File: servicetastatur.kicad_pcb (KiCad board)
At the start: 2 copper layers, 113.9 x 58 mm, 70 parts, among them J1 Conn_01x02, J2 LCD, J3 Automat, J4 Tasten, J5 Conn_01x03_Pin, J6 Conn_01x03_Pin, Q1 2N3904, U1 74HC238, U17 TL7705A, U18 MC34063AP, U2 74HC00, U3 27C128, U4 80C31, U5 74LS573, U6 74HC4094, U7 74HC4094, U8 74HC165, U9 24CS16, Y1 11.059

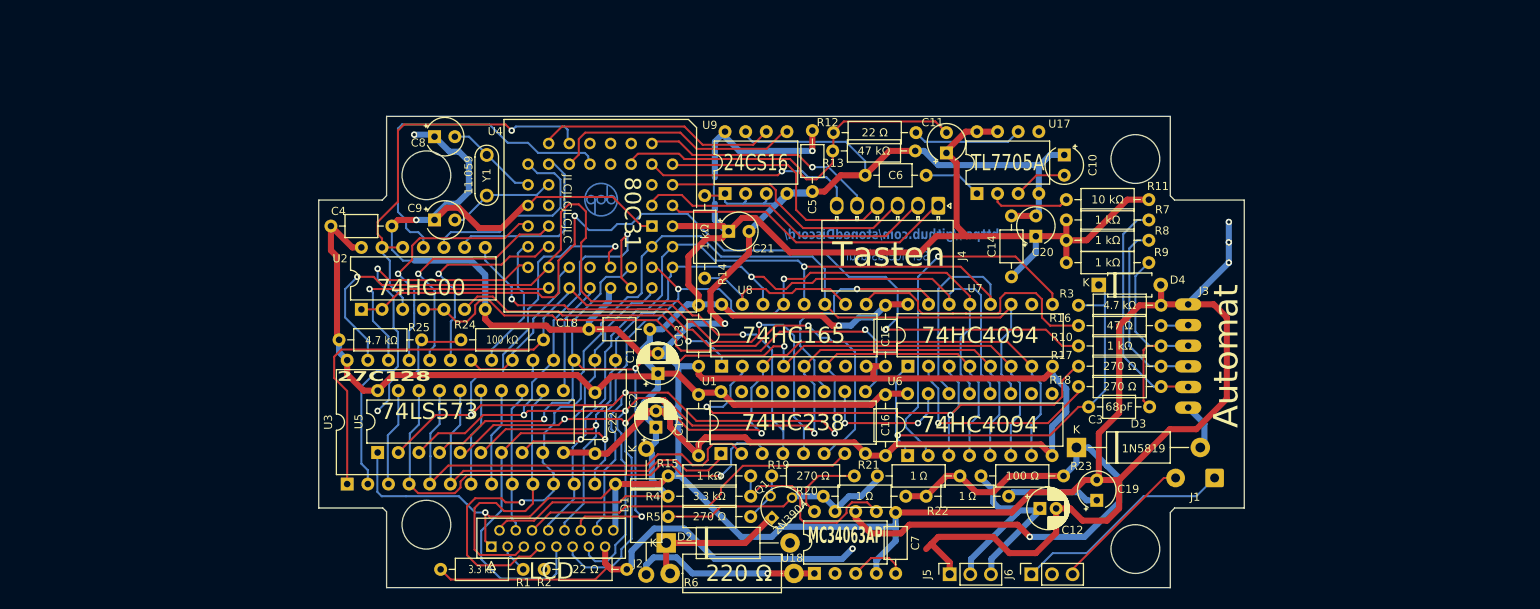
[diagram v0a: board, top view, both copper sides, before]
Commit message: kompakt
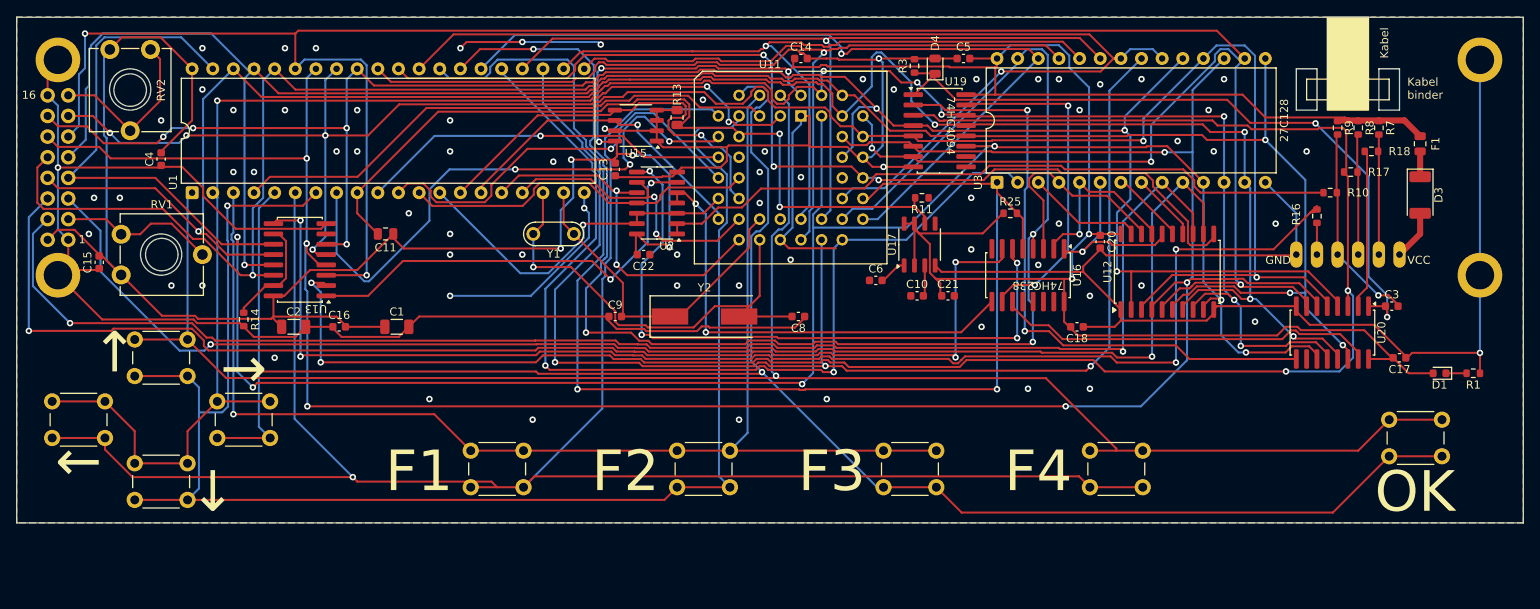
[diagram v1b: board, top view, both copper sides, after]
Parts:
- removed C12: C_Polarized, Capacitor_THT:CP_Radial_D5.0mm_P2.00mm
- removed C19: C, Capacitor_THT:CP_Radial_Tantal_D4.5mm_P2.50mm
- removed C7: C, Capacitor_THT:C_Axial_L3.8mm_D2.6mm_P7.50mm_Horizontal
- removed D2: D, Diode_THT:D_DO-15_P15.24mm_Horizontal
- removed J1: Conn_01x02, Connector_Wire:SolderWire-0.5sqmm_1x02_P4.8mm_D0.9mm_OD2.3mm
- removed J4: Tasten, adp:FFC_1x06_P2.50mm_Horizontal
- removed J5, J6: Conn_01x03_Pin, Connector_PinSocket_2.54mm:PinSocket_1x03_P2.54mm_Vertical
- removed Q1: 2N3904, adp:TO-92
- removed R12, R2: 22 Ω, Resistor_THT:R_Axial_DIN0207_L6.3mm_D2.5mm_P10.16mm_Horizontal
- removed R15: 1 kΩ, Resistor_THT:R_Axial_DIN0207_L6.3mm_D2.5mm_P10.16mm_Horizontal
- removed R19, R5: 270 Ω, Resistor_THT:R_Axial_DIN0207_L6.3mm_D2.5mm_P10.16mm_Horizontal
- removed R20, R21, R22: 1 Ω, Resistor_THT:R_Axial_DIN0207_L6.3mm_D2.5mm_P10.16mm_Horizontal
- removed R23: 100 Ω, Resistor_THT:R_Axial_DIN0207_L6.3mm_D2.5mm_P10.16mm_Horizontal
- removed R24: 100 kΩ, Resistor_THT:R_Axial_DIN0207_L6.3mm_D2.5mm_P10.16mm_Horizontal
- removed R4: 3.3 kΩ, Resistor_THT:R_Axial_DIN0207_L6.3mm_D2.5mm_P10.16mm_Horizontal
- removed R6: 220 Ω, Resistor_THT:R_Axial_DIN0414_L11.9mm_D4.5mm_P15.24mm_Horizontal
- removed U18: MC34063AP, Package_DIP:DIP-8_W7.62mm
- removed U4: 80C31, Package_LCC:PLCC-44_THT-Socket
- removed U5: 74LS573, Package_DIP:DIP-20_W7.62mm
- removed U6, U7: 74HC4094, Package_DIP:DIP-16_W7.62mm
- removed U8: 74HC165, Package_DIP:DIP-16_W7.62mm
- removed U9: 24CS16, Package_DIP:DIP-8_W7.62mm
- added F1: Fuse, Fuse:Fuse_0805_2012Metric, F.Cu at (185.4, 34.6)
- added RV1: Kontrast, Potentiometer_THT:Potentiometer_ACP_CA9-V10_Vertical_Hole, F.Cu at (25.6, 50.8)
- added RV2: Helligkeit, Potentiometer_THT:Potentiometer_ACP_CA9-V10_Vertical_Hole, F.Cu at (24.2, 23.0)
- added SW1: OK, Button_Switch_THT:SW_PUSH_6mm, F.Cu at (181.6, 68.6)
- added SW2: →, Button_Switch_THT:SW_PUSH_6mm, F.Cu at (37.4, 66.3)
- added SW3: F3, Button_Switch_THT:SW_PUSH_6mm, F.Cu at (119.4, 72.4)
- added SW4: F4, Button_Switch_THT:SW_PUSH_6mm, F.Cu at (144.8, 72.4)
- added SW5: ←, Button_Switch_THT:SW_PUSH_6mm, F.Cu at (17.1, 66.3)
- added SW6: F1, Button_Switch_THT:SW_PUSH_6mm, F.Cu at (68.6, 72.4)
- added SW7: ↑, Button_Switch_THT:SW_PUSH_6mm, F.Cu at (27.2, 58.7)
- added SW8: ↓, Button_Switch_THT:SW_PUSH_6mm, F.Cu at (27.2, 74.0)
- added SW9: F2, Button_Switch_THT:SW_PUSH_6mm, F.Cu at (94.0, 72.4)
- added U11: 80C31, Package_LCC:PLCC-44_THT-Socket, F.Cu at (109.2, 31.2)
- added U12: 74LS573, Package_SO:SOIC-20W_7.5x12.8mm_P1.27mm, F.Cu at (154.3, 50.4)
- added U13: 74HC165, Package_SO:SOIC-16W_5.3x10.2mm_P1.27mm, F.Cu at (47.5, 48.9)
- added U15: 24CS16, Package_SO:SO-8_3.9x4.9mm_P1.27mm, F.Cu at (88.9, 32.4)
- added U16: 74HC238, Package_SO:SOIC-16W_5.3x10.2mm_P1.27mm, F.Cu at (137.2, 50.8)
- added U19: 74HC4094, Package_SO:SOIC-16W_5.3x10.2mm_P1.27mm, F.Cu at (126.3, 33.0)
- added U20: 74HC4094, Package_SO:SOIC-16W_5.3x10.2mm_P1.27mm, F.Cu at (174.6, 57.9)
- added Y2: 11.059, Crystal:Crystal_SMD_HC49-SD, F.Cu at (97.3, 55.9)
- C1: value C_Polarized -> 1uF; footprint Capacitor_THT:CP_Radial_D5.0mm_P2.50mm -> Capacitor_SMD:C_1206_3216Metric
- C10: value C -> 0,1uF; footprint Capacitor_THT:CP_Radial_Tantal_D4.5mm_P2.50mm -> Capacitor_SMD:C_0603_1608Metric
- C11: footprint Capacitor_THT:CP_Radial_Tantal_D4.5mm_P2.50mm -> Capacitor_SMD:C_0805_2012Metric
- C13, C14, C15, C16, C17, C18, C22, C5: value C -> 100nF; footprint Capacitor_THT:C_Axial_L3.8mm_D2.6mm_P7.50mm_Horizontal -> Capacitor_SMD:C_0603_1608Metric
- C2: value C_Polarized -> 1uF; footprint Capacitor_THT:CP_Radial_D5.0mm_P2.00mm -> Capacitor_SMD:C_1206_3216Metric
- C20, C21: value C -> 100nF; footprint Capacitor_THT:CP_Radial_Tantal_D4.5mm_P2.50mm -> Capacitor_SMD:C_0603_1608Metric
- C3: footprint Capacitor_THT:C_Axial_L3.8mm_D2.6mm_P7.50mm_Horizontal -> Capacitor_SMD:C_0603_1608Metric
- C4: value C -> 1uF; footprint Capacitor_THT:C_Axial_L3.8mm_D2.6mm_P7.50mm_Horizontal -> Capacitor_SMD:C_0603_1608Metric
- C6: value C -> 0,1uF; footprint Capacitor_THT:C_Axial_L3.8mm_D2.6mm_P7.50mm_Horizontal -> Capacitor_SMD:C_0603_1608Metric
- C8, C9: value C -> 33pF; footprint Capacitor_THT:CP_Radial_Tantal_D4.5mm_P2.50mm -> Capacitor_SMD:C_0603_1608Metric
- D1: value 1N5819 -> LED; footprint adp:D_DO-15_P15mm_Horizontal -> LED_SMD:LED_0603_1608Metric
- D3: footprint Diode_THT:D_DO-15_P15.24mm_Horizontal -> Diode_SMD:D_2010_5025Metric
- D4: footprint Diode_THT:D_A-405_P7.62mm_Horizontal -> Diode_SMD:D_0805_2012Metric
- J2: value LCD -> Conn_02x08_Odd_Even_MountingPin; footprint adp:FFC_2x08_P1mm_Vertical -> ConnPad:LCDdisplay
- R1: value 3.3 kΩ -> 470; footprint Resistor_THT:R_Axial_DIN0207_L6.3mm_D2.5mm_P10.16mm_Horizontal -> Resistor_SMD:R_0603_1608Metric
- R10, R11, R14, R16, R17, R18, R25, R3, R7, R8, R9: footprint Resistor_THT:R_Axial_DIN0207_L6.3mm_D2.5mm_P10.16mm_Horizontal -> Resistor_SMD:R_0603_1608Metric
- R13: footprint Resistor_THT:R_Axial_DIN0207_L6.3mm_D2.5mm_P10.16mm_Horizontal -> Resistor_SMD:R_0805_2012Metric
- U1: value 74HC238 -> ~; footprint Package_DIP:DIP-16_W7.62mm -> Package_DIP:DIP-40_W15.24mm
- U17: footprint Package_DIP:DIP-8_W7.62mm -> Package_SO:SO-8_3.9x4.9mm_P1.27mm
- U2: footprint Package_DIP:DIP-14_W7.62mm -> Package_SO:SOIC-14_3.9x8.7mm_P1.27mm
- moved R1 129.4 mm to (192.0, 62.9), turned to 180 degrees
- moved D1 98.1 mm to (187.8, 62.9), turned to 180 degrees
- moved C15 97.6 mm to (22.9, 49.2)
- moved U3 88.2 mm to (133.3, 39.4)
- moved C17 87.1 mm to (182.9, 61.0), turned to 180 degrees
- moved R25 84.1 mm to (135.0, 43.2)
- moved U1 72.6 mm to (34.3, 40.6)
- moved C11 69.7 mm to (58.1, 45.7), turned to 180 degrees
- moved C16 69.1 mm to (52.4, 57.1), turned to 0 degrees
- moved C18 60.1 mm to (143.2, 57.1), turned to 180 degrees
- moved R14 57.0 mm to (40.6, 56.2), turned to -90 degrees
- moved J2 55.8 mm to (101.8, 37.5), turned to 0 degrees
- moved D3 52.5 mm to (185.4, 40.9), turned to -90 degrees
- moved C8 49.9 mm to (108.9, 55.9), turned to 180 degrees
- moved C2 46.3 mm to (46.8, 57.1), turned to 0 degrees
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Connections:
- C8 pad 2: Net-(U4-XTAL2) -> Net-(U1-XTAL2)
- C9 pad 2: Net-(U4-XTAL1) -> Net-(U1-XTAL1)
- D1 pad 1: VCC -> Net-(D1-K)
- D1 pad 2: Net-(D1-A) -> VCC
- J2 pad 15: VCC -> /Helligkeit
- J2 pad 3: Net-(J2-Pin_3) -> /Kontrast
- J2 pad 6: Net-(J2-Pin_6) -> /LCD_EN
- R1 pad 1: VCC -> GND
- R1 pad 2: Net-(J2-Pin_3) -> Net-(D1-K)
- R11 pad 1: Net-(U17-~{RESIN}) -> GND
- R11 pad 2: VCC -> RESET
- R25 pad 2: Net-(R24-Pad1) -> A15
- U1 pad 1: A4 -> Net-(U1-P1.0)
- U1 pad 10: Net-(U1-Y5) -> unconnected-(U1-P3.0/RxD-Pad10)
- U1 pad 11: Net-(U1-Y4) -> unconnected-(U1-P3.1/TxD-Pad11)
- U1 pad 12: unconnected-(U1-Y3-Pad12) -> Net-(U1-P3.2/INT0)
- U1 pad 13: unconnected-(U1-Y2-Pad13) -> Net-(U1-P3.3/INT1)
- U1 pad 14: unconnected-(U1-Y1-Pad14) -> SDA
- U1 pad 15: unconnected-(U1-Y0-Pad15) -> SCL
- U1 pad 16: VCC -> Net-(U1-P3.6/WR)
- U1 pad 2: A5 -> Net-(U1-P1.1)
- U1 pad 3: A6 -> Net-(U1-P1.2)
- U1 pad 4: A14 -> unconnected-(U1-P1.3-Pad4)
- U1 pad 5: A15 -> Net-(U1-P1.4)
- U1 pad 6: Net-(U1-E3) -> Net-(U1-P1.5)
- U1 pad 7: Net-(J2-Pin_6) -> Net-(U1-P1.6)
- U1 pad 8: GND -> unconnected-(U1-P1.7-Pad8)
- U1 pad 9: Net-(U1-Y6) -> RESET
- U17 pad 2: Net-(U17-~{RESIN}) -> VCC
- U17 pad 6: Net-(U17-RESET) -> RESET
- U2 pad 10: Net-(U4-P3.6/WR) -> Net-(U1-P3.6/WR)
- U2 pad 11: Net-(U4-P3.2/INT0) -> Net-(U1-P3.2/INT0)
- U2 pad 12: Net-(U4-P3.3/INT1) -> Net-(U1-P3.3/INT1)
- U2 pad 13: Net-(U4-P3.3/INT1) -> Net-(U1-P3.3/INT1)
- U2 pad 3: Net-(U4-P3.3/INT1) -> Net-(U1-P3.3/INT1)
- U2 pad 4: Net-(U1-Y6) -> Net-(U16-Y6)
- U2 pad 5: Net-(U1-Y6) -> Net-(U16-Y6)
- U2 pad 8: Net-(U1-E3) -> Net-(U16-E3)
- U2 pad 9: Net-(U4-P3.7/RD) -> Net-(U1-P3.7/RD)
- U3 pad 2: Net-(U3-A12) -> Net-(U1-P2.4/A12)
- U3 pad 20: Net-(U3-~{CE}) -> Net-(U1-PSEN)
- U3 pad 21: Net-(U3-A10) -> Net-(U1-P2.2/A10)
- U3 pad 22: Net-(U3-~{CE}) -> Net-(U1-PSEN)
- U3 pad 23: Net-(U3-A11) -> Net-(U1-P2.3/A11)
- U3 pad 24: Net-(U3-A9) -> Net-(U1-P2.1/A9)
- U3 pad 25: Net-(U3-A8) -> Net-(U1-P2.0/A8)
- U3 pad 26: Net-(U3-A13) -> Net-(U1-P2.5/A13)
- Y1 pad 1: Net-(U4-XTAL1) -> Net-(U1-XTAL1)
- Y1 pad 2: Net-(U4-XTAL2) -> Net-(U1-XTAL2)
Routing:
- net Net-(U1-P1.5): track 0.00 -> 243.4 mm, vias 0 -> 1
- net Net-(U1-P1.4): track 0.00 -> 236.4 mm, vias 0 -> 2
- net Net-(U1-P1.0): track 0.00 -> 226.3 mm, vias 0 -> 1
- net Net-(U1-P1.6): track 0.00 -> 190.0 mm, vias 0 -> 1
- net D4: track 146.1 -> 312.2 mm, vias 3 -> 5
- net Net-(U1-P2.2/A10): track 0.00 -> 164.4 mm, vias 0 -> 3
- net Net-(U1-P1.2): track 0.00 -> 161.1 mm, vias 0 -> 1
- net A1: track 18.0 -> 177.9 mm, vias 0 -> 2
- net CLOCK: track 69.8 -> 227.9 mm, vias 2 -> 4
- net D5: track 140.3 -> 297.1 mm, vias 4 -> 6
- net /LCD_EN: track 0.00 -> 153.0 mm, vias 0 -> 3
- net D0: track 130.0 -> 279.2 mm, vias 1 -> 6
- net Net-(U1-P1.1): track 0.00 -> 149.2 mm, vias 0 -> 3
- net A0: track 34.6 -> 176.2 mm, vias 0 -> 2
- net D3: track 114.5 -> 252.3 mm, vias 2 -> 4
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- added copper zone on B.Cu, net GND
- added copper zone on F.Cu, net GND
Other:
- board size 113.9 x 58 mm -> 185.4 x 62.2 mm
- board text added: "1"
- board text added: "16"
- board text added: "GND"
- board text added: "Kabel"
- board text added: "Kabel binder"
- board text added: "VCC"
- board text removed: "JLCJLCJLCJLC"
- board text removed: "https://github.com/stonedDiscord/"
- board text removed: "servicetastatur"
